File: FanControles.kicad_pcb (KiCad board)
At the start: 2 copper layers, 29 x 18 mm, 5 parts, among them P1 24v Fan, P2 24v, P3 100k NTC, Q1 BSH103BKR

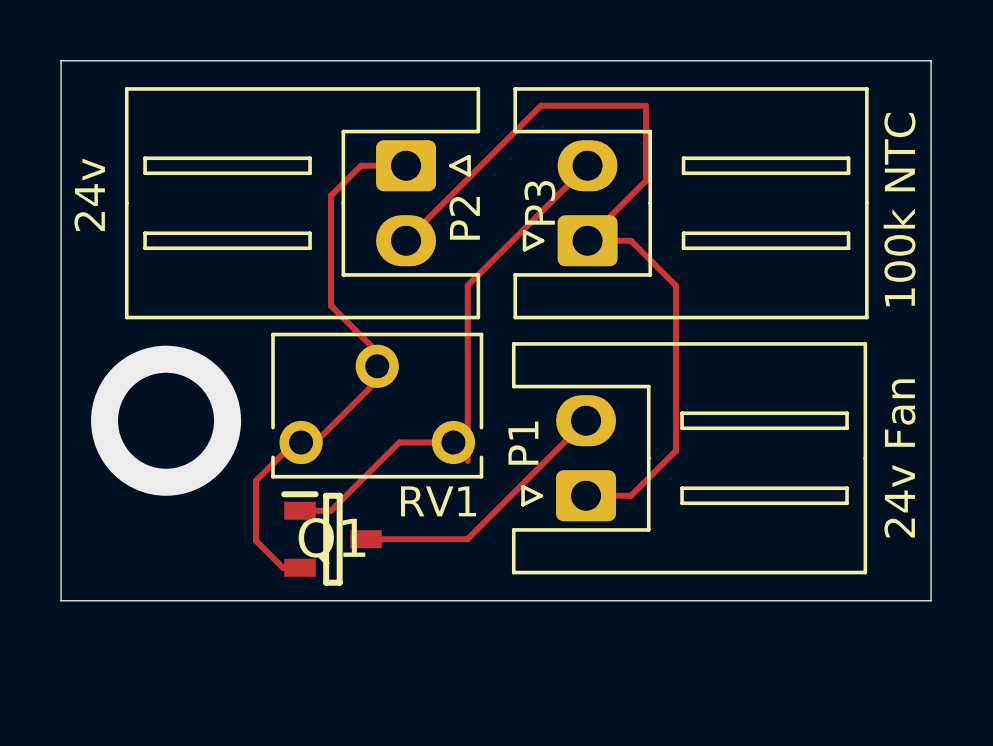
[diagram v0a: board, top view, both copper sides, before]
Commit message: bk
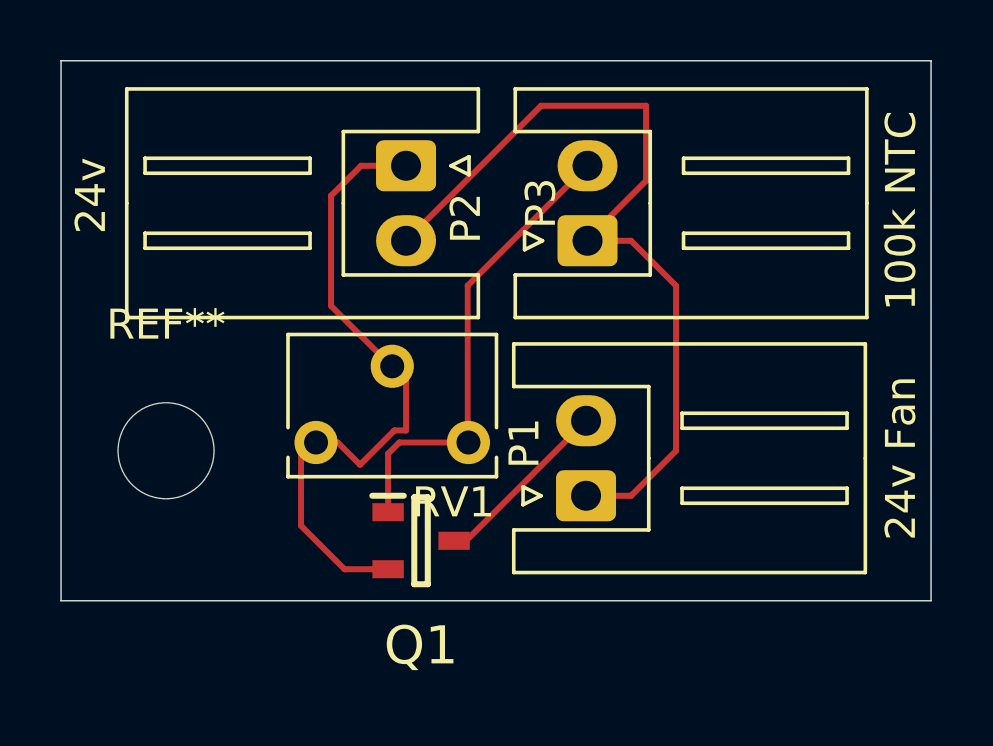
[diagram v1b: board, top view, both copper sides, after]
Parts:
- added REF**: MountingHole_3.2mm_M3, MountingHole:MountingHole_3.2mm_M3, F.Cu at (137.0, 89.5)
- moved Q1 2.94 mm to (145.5, 92.5)
- moved RV1 0.50 mm to (142.0, 89.2)
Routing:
- net /Fan: track 9.14 -> 6.06 mm
- net GND: track 19.5 -> 22.3 mm
- net Net-(Q1-G): track 17.9 -> 16.3 mm
- net (no net): vias 1 -> 0
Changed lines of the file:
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@@
 			(outputformat 1)
 			(mirror no)
-			(drillshape 1)
+			(drillshape 0)
 			(scaleselection 1)
-			(outputdirectory "")
+			(outputdirectory "gerbers/")
 		)
 	)
@@
 		)
 	)
+	(footprint "MountingHole:MountingHole_3.2mm_M3"
+		(layer "F.Cu")
+		(at 137 89.5)
+		(descr "Mounting Hole 3.2mm, no annular, M3")
+		(tags "mounting hole 3.2mm no annular m3")
+		(property "Reference" "REF**"
+			(at 0 -4.2 0)
+			(layer "F.SilkS")
+			(effects
+				(font
+					(size 1 1)
+					(thickness 0.15)
+				)
+			)
+		)
+		(property "Value" "MountingHole_3.2mm_M3"
+			(at 0 4.2 0)
+			(layer "F.Fab")
+			(effects
+				(font
+					(size 1 1)
+					(thickness 0.15)
+				)
+			)
+		)
+		(property "Datasheet" ""
+			(at 0 0 0)
+			(unlocked yes)
+			(layer "F.Fab")
+			(hide yes)
+			(effects
+				(font
+					(size 1.27 1.27)
+					(thickness 0.15)
+				)
+			)
+		)
+		(property "Description" ""
+			(at 0 0 0)
+			(unlocked yes)
+			(layer "F.Fab")
+			(hide yes)
+			(effects
+				(font
+					(size 1.27 1.27)
+					(thickness 0.15)
+				)
+			)
+		)
+		(attr exclude_from_pos_files exclude_from_bom)
+		(fp_circle
+			(center 0 0)
+			(end 3.2 0)
+			(stroke
+				(width 0.15)
+				(type solid)
+			)
+			(fill no)
+			(layer "Cmts.User")
+		)
+		(fp_circle
+			(center 0 0)
+			(end 3.45 0)
+			(stroke
+				(width 0.05)
+				(type solid)
+			)
+			(fill no)
+			(layer "F.CrtYd")
+		)
+		(fp_text user "${REFERENCE}"
+			(at 0 0 0)
+			(layer "F.Fab")
+			(effects
+				(font
+					(size 1 1)
+					(thickness 0.15)
+				)
+			)
+		)
+		(pad "" np_thru_hole circle
+			(at 0 0)
+			(size 3.2 3.2)
+			(drill 3.2)
+			(layers "*.Cu" "*.Mask")
+		)
+		(embedded_fonts no)
+	)
 	(footprint "Connector_JST:JST_XH_S2B-XH-A_1x02_P2.50mm_Horizontal"
 		(layer "F.Cu")
@@
 	(footprint "BSH:SOT95P230X110-3N"
 		(layer "F.Cu")
-		(at 142.5625 92.45)
+		(at 145.5 92.5)
 		(descr "SOT23 Nexperia")
 		(tags "MOSFET (N-Channel)")
 		(property "Reference" "Q1"
-			(at 0 0 0)
+			(at 0 3.5 0)
 			(layer "F.SilkS")
 			(effects
@@
 		)
 		(property "Value" "BSH103BKR"
-			(at 0 0 -0)
+			(at 0 0 0)
 			(layer "B.SilkS")
 			(effects
@@
 		)
 		(fp_text user "${REFERENCE}"
-			(at 0 0 0)
+			(at 3.1 3.5 0)
 			(layer "F.Fab")
 			(effects
@@
 	(footprint "Potentiometer_THT:Potentiometer_Bourns_3266W_Vertical"
 		(layer "F.Cu")
-		(at 141.5 89.225 180)
+		(at 142 89.225 180)
 		(descr "Potentiometer, vertical, Bourns 3266W, https://www.bourns.com/docs/Product-Datasheets/3266.pdf")
 		(tags "Potentiometer vertical Bourns 3266W")
@@
 	(dimension
 		(type orthogonal)
-		(layer "Edge.Cuts")
+		(layer "User.1")
 		(pts
 			(xy 162.5 76.5) (xy 133.5 76.5)
@@
 		(gr_text "29"
 			(at 148 72.85 0)
-			(layer "Edge.Cuts")
+			(layer "User.1")
 			(effects
 				(font
@@
 	(dimension
 		(type orthogonal)
-		(layer "Edge.Cuts")
+		(layer "User.1")
 		(pts
 			(xy 162.5 94.5) (xy 162.5 76.5)
@@
 		(gr_text "18"
 			(at 165.35 85.5 90)
-			(layer "Edge.Cuts")
-			(effects
-				(font
-					(size 1 1)
-					(thickness 0.15)
-				)
-			)
-		)
-	)
-	(via
-		(at 137 88.5)
-		(size 5)
-		(drill 3.2)
-		(layers "F.Cu" "B.Cu")
-		(free yes)
-		(net 0)
+			(layer "User.1")
+			(effects
+				(font
+					(size 1 1)
+					(thickness 0.15)
+				)
+			)
+		)
 	)
 	(segment
@@
 	)
 	(segment
-		(start 147.05 92.45)
-		(end 151 88.5)
+		(start 151 88.5)
+		(end 147 92.5)
 		(width 0.2)
 		(layer "F.Cu")
@@
 	)
 	(segment
-		(start 143.5 92.45)
-		(end 147.05 92.45)
+		(start 147 92.5)
+		(end 146.6 92.5)
 		(width 0.2)
 		(layer "F.Cu")
@@
 	)
 	(segment
-		(start 140 90.5)
-		(end 140 92.5)
+		(start 141.5 92)
+		(end 141.5 89.225)
 		(width 0.2)
 		(layer "F.Cu")
@@
 	)
 	(segment
+		(start 142.5 84.67)
+		(end 142.5 81)
+		(width 0.2)
+		(layer "F.Cu")
+		(net 3)
+	)
+	(segment
+		(start 145 87.17)
+		(end 142.5 84.67)
+		(width 0.2)
+		(layer "F.Cu")
+		(net 3)
+	)
+	(segment
+		(start 144.6089 88.824)
+		(end 145 88.824)
+		(width 0.2)
+		(layer "F.Cu")
+		(net 3)
+	)
+	(segment
+		(start 143.5 80)
+		(end 145 80)
+		(width 0.2)
+		(layer "F.Cu")
+		(net 3)
+	)
+	(segment
+		(start 142.725 89.225)
+		(end 143.46645 89.96645)
+		(width 0.2)
+		(layer "F.Cu")
+		(net 3)
+	)
+	(segment
+		(start 144.4 93.45)
+		(end 142.95 93.45)
+		(width 0.2)
+		(layer "F.Cu")
+		(net 3)
+	)
+	(segment
+		(start 145 88.824)
+		(end 145 87.17)
+		(width 0.2)
+		(layer "F.Cu")
+		(net 3)
+	)
+	(segment
+		(start 143.46645 89.96645)
+		(end 144.6089 88.824)
+		(width 0.2)
+		(layer "F.Cu")
+		(net 3)
+	)
+	(segment
+		(start 142.95 93.45)
+		(end 141.5 92)
+		(width 0.2)
+		(layer "F.Cu")
+		(net 3)
+	)
+	(segment
 		(start 142.5 81)
-		(end 142.5 84.67)
+		(end 143.5 80)
 		(width 0.2)
 		(layer "F.Cu")
@@
 	)
 	(segment
-		(start 145 80)
-		(end 143.5 80)
+		(start 141.5 89.225)
+		(end 142.725 89.225)
 		(width 0.2)
 		(layer "F.Cu")
@@
 	)
 	(segment
-		(start 141.275 89.225)
-		(end 140 90.5)
-		(width 0.2)
-		(layer "F.Cu")
-		(net 3)
-	)
-	(segment
-		(start 140 92.5)
-		(end 140.9 93.4)
-		(width 0.2)
-		(layer "F.Cu")
-		(net 3)
-	)
-	(segment
-		(start 141.975 89.225)
-		(end 141.275 89.225)
-		(width 0.2)
-		(layer "F.Cu")
-		(net 3)
-	)
-	(segment
-		(start 143.5 80)
-		(end 142.5 81)
-		(width 0.2)
-		(layer "F.Cu")
-		(net 3)
-	)
-	(segment
-		(start 140.9 93.4)
-		(end 141.625 93.4)
-		(width 0.2)
-		(layer "F.Cu")
-		(net 3)
-	)
-	(segment
-		(start 144.515 86.685)
-		(end 141.975 89.225)
-		(width 0.2)
-		(layer "F.Cu")
-		(net 3)
-	)
-	(segment
-		(start 142.5 84.67)
-		(end 144.515 86.685)
-		(width 0.2)
-		(layer "F.Cu")
-		(net 3)
-	)
-	(segment
-		(start 142.5 91.5)
-		(end 144.775 89.225)
-		(width 0.2)
-		(layer "F.Cu")
-		(net 4)
-	)
-	(segment
-		(start 141.625 91.5)
-		(end 142.5 91.5)
+		(start 144.775 89.225)
+		(end 147.055 89.225)
 		(width 0.2)
 		(layer "F.Cu")
@@
 	)
 	(segment
+		(start 144.4 91.55)
+		(end 144.4 89.6)
+		(width 0.2)
+		(layer "F.Cu")
+		(net 4)
+	)
+	(segment
+		(start 144.4 89.6)
+		(end 144.775 89.225)
+		(width 0.2)
+		(layer "F.Cu")
+		(net 4)
+	)
+	(segment
 		(start 151.05 80)
 		(end 147.055 83.995)
@@
 		(width 0.2)
 		(layer "F.Cu")
-		(net 4)
-	)
-	(segment
-		(start 144.775 89.225)
-		(end 147.055 89.225)
-		(width 0.2)
-		(layer "F.Cu")
